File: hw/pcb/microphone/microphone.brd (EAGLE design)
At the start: 15 x 15 mm, 17 parts

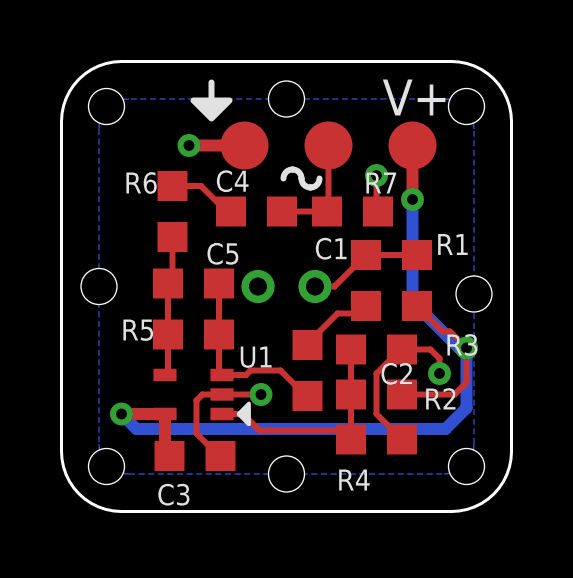
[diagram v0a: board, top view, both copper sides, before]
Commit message: Final tweaks and CAM output for all three boards
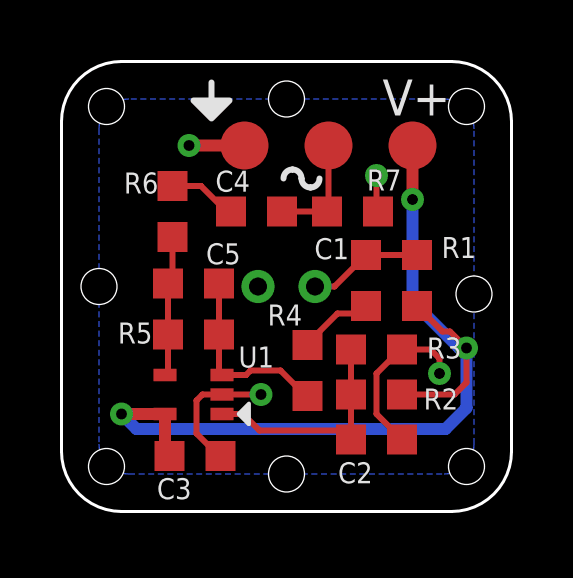
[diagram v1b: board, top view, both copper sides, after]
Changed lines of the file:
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@@
 <layer number="27" name="tValues" color="7" fill="1" visible="no" active="yes"/>
 <layer number="28" name="bValues" color="7" fill="1" visible="no" active="yes"/>
-<layer number="29" name="tStop" color="7" fill="3" visible="no" active="yes"/>
-<layer number="30" name="bStop" color="7" fill="6" visible="no" active="yes"/>
-<layer number="31" name="tCream" color="7" fill="4" visible="no" active="yes"/>
-<layer number="32" name="bCream" color="7" fill="5" visible="no" active="yes"/>
+<layer number="29" name="tStop" color="7" fill="3" visible="yes" active="yes"/>
+<layer number="30" name="bStop" color="7" fill="6" visible="yes" active="yes"/>
+<layer number="31" name="tCream" color="7" fill="4" visible="yes" active="yes"/>
+<layer number="32" name="bCream" color="7" fill="5" visible="yes" active="yes"/>
 <layer number="33" name="tFinish" color="6" fill="3" visible="no" active="yes"/>
 <layer number="34" name="bFinish" color="6" fill="6" visible="no" active="yes"/>
@@
 <attribute name="NOSTUFF" value="" x="11.85" y="7.7" size="0.9" layer="27" ratio="10" rot="R270" display="off"/>
 <attribute name="COST_X500" value=".00514" x="11.85" y="7.7" size="0.9" layer="27" ratio="10" rot="R270" display="off"/>
-<attribute name="NAME" x="12.47" y="8.55" size="0.7" layer="21" font="vector"/>
+<attribute name="NAME" x="12.67" y="8.45" size="0.7" layer="21" font="vector"/>
 <attribute name="NAME" x="10.85" y="6.43" size="1" layer="105" font="vector" rot="R270"/>
 </element>
@@
 <attribute name="NOSTUFF" value="" x="10.5" y="5.4" size="0.9" layer="27" ratio="10" rot="R180" display="off"/>
 <attribute name="COST_X500" value=".00382" x="10.5" y="5.4" size="0.9" layer="27" ratio="10" rot="R180" display="off"/>
-<attribute name="NAME" x="13.93" y="5.9" size="0.7" layer="21" font="vector" rot="R180"/>
+<attribute name="NAME" x="13.33" y="5.8" size="0.7" layer="21" font="vector" rot="R180"/>
 <attribute name="NAME" x="9.23" y="6.4" size="1" layer="105" font="vector" rot="R180"/>
 </element>
@@
 <attribute name="NOSTUFF" value="" x="10.5" y="2.4" size="0.9" layer="27" ratio="10" rot="R180" display="off"/>
 <attribute name="COST_X500" value="0.06626" x="10.5" y="2.4" size="0.9" layer="27" ratio="10" rot="R180" display="off"/>
-<attribute name="NAME" x="11.77" y="4.94" size="0.7" layer="21" font="vector" rot="R180"/>
+<attribute name="NAME" x="10.37" y="1.64" size="0.7" layer="21" font="vector" rot="R180"/>
 </element>
 <element name="C3" library="wedfestdress" package="CAP_0603" value="" x="4.45" y="1.85" smashed="yes">
@@
 <attribute name="NOSTUFF" value="" x="4.45" y="1.85" size="0.9" layer="27" ratio="10" display="off"/>
 <attribute name="COST_X500" value="0.0154" x="4.45" y="1.85" size="0.9" layer="27" ratio="10" display="off"/>
-<attribute name="NAME" x="3.18" y="0.21" size="0.7" layer="21" font="vector"/>
+<attribute name="NAME" x="3.18" y="0.41" size="0.7" layer="21" font="vector"/>
 </element>
 <element name="R4" library="wedfestdress" package="RES_0603" value="" x="8.2" y="4.7" smashed="yes" rot="R270">
@@
 <attribute name="NOSTUFF" value="" x="8.2" y="4.7" size="0.9" layer="27" ratio="10" rot="R270" display="off"/>
 <attribute name="COST_X500" value="0.00278" x="8.2" y="4.7" size="0.9" layer="27" ratio="10" rot="R270" display="off"/>
-<attribute name="NAME" x="9.17" y="0.7" size="0.7" layer="21" font="vector"/>
+<attribute name="NAME" x="6.87" y="6.2" size="0.7" layer="21" font="vector"/>
 <attribute name="NAME" x="7.2" y="3.43" size="1" layer="105" font="vector" rot="R270"/>
 </element>
@@
 <attribute name="NOSTUFF" value="" x="4.4" y="5.9" size="0.9" layer="27" ratio="10" rot="R180" display="off"/>
 <attribute name="COST_X500" value=".006" x="4.4" y="5.9" size="0.9" layer="27" ratio="10" rot="R180" display="off"/>
-<attribute name="NAME" x="3.13" y="6.4" size="0.7" layer="21" font="vector" rot="R180"/>
+<attribute name="NAME" x="3.03" y="6.3" size="0.7" layer="21" font="vector" rot="R180"/>
 <attribute name="NAME" x="3.13" y="6.9" size="1" layer="105" font="vector" rot="R180"/>
 </element>
@@
 <attribute name="NOSTUFF" value="" x="9.7" y="10" size="0.9" layer="27" ratio="10" rot="R180" display="off"/>
 <attribute name="COST_X500" value=".00316" x="9.7" y="10" size="0.9" layer="27" ratio="10" rot="R180" display="off"/>
-<attribute name="NAME" x="11.23" y="11.3" size="0.7" layer="21" font="vector" rot="R180"/>
+<attribute name="NAME" x="11.33" y="11.4" size="0.7" layer="21" font="vector" rot="R180"/>
 <attribute name="NAME" x="8.43" y="11" size="1" layer="105" font="vector" rot="R180"/>
 </element>
